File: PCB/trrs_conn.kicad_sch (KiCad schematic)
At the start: 4 parts, among them J501 AudioJack4, J502 AudioJack4, U501 USBLC6-2SC6, U502 USBLC6-2SC6

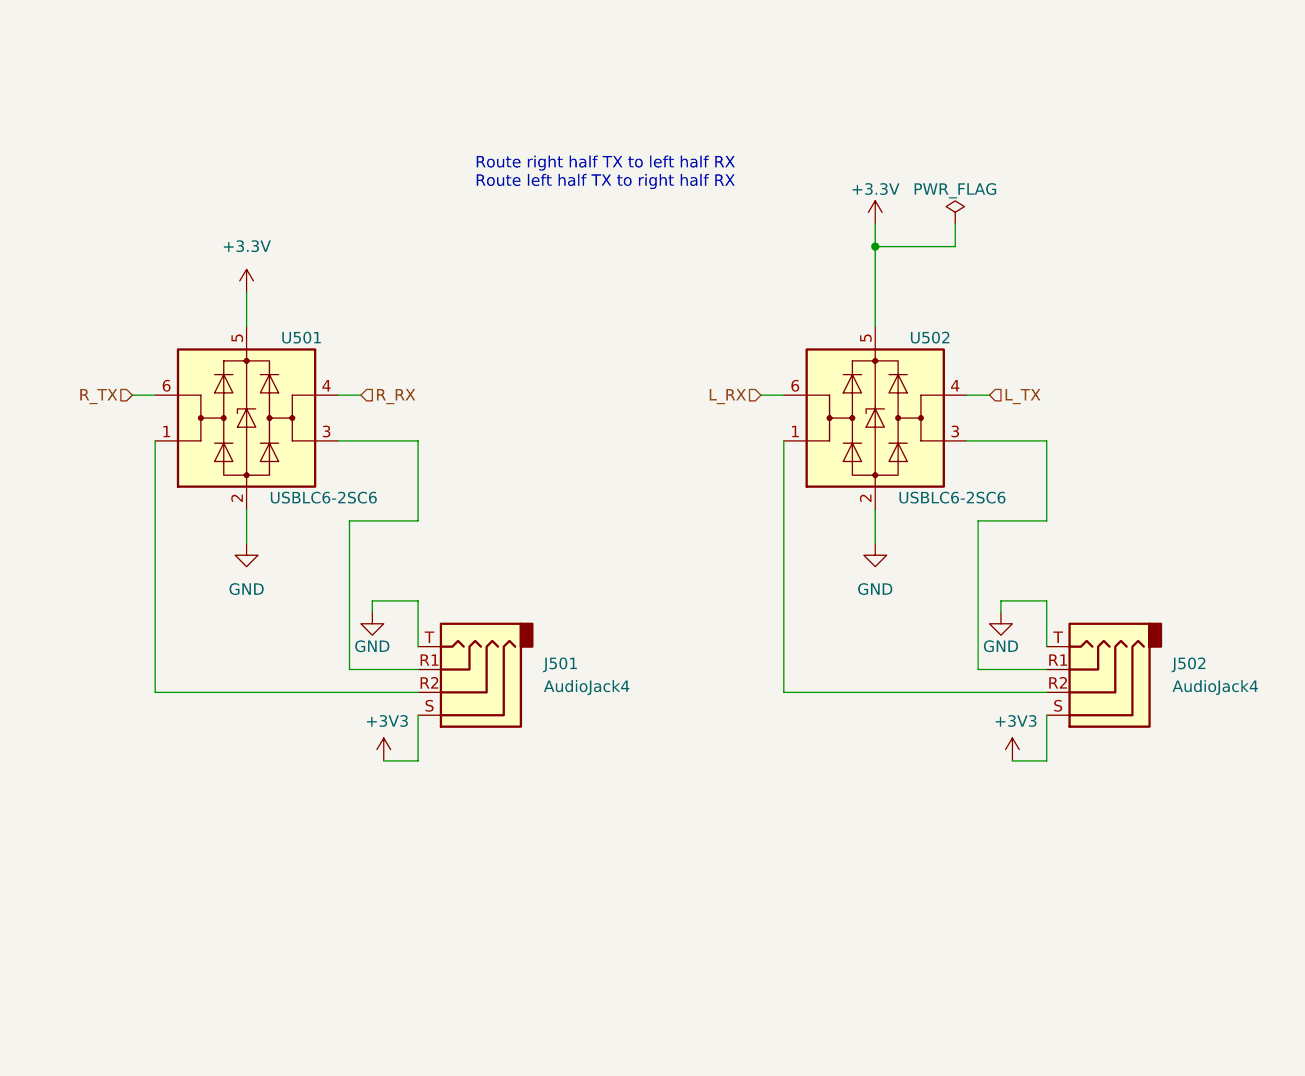
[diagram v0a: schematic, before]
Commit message: Update net labels
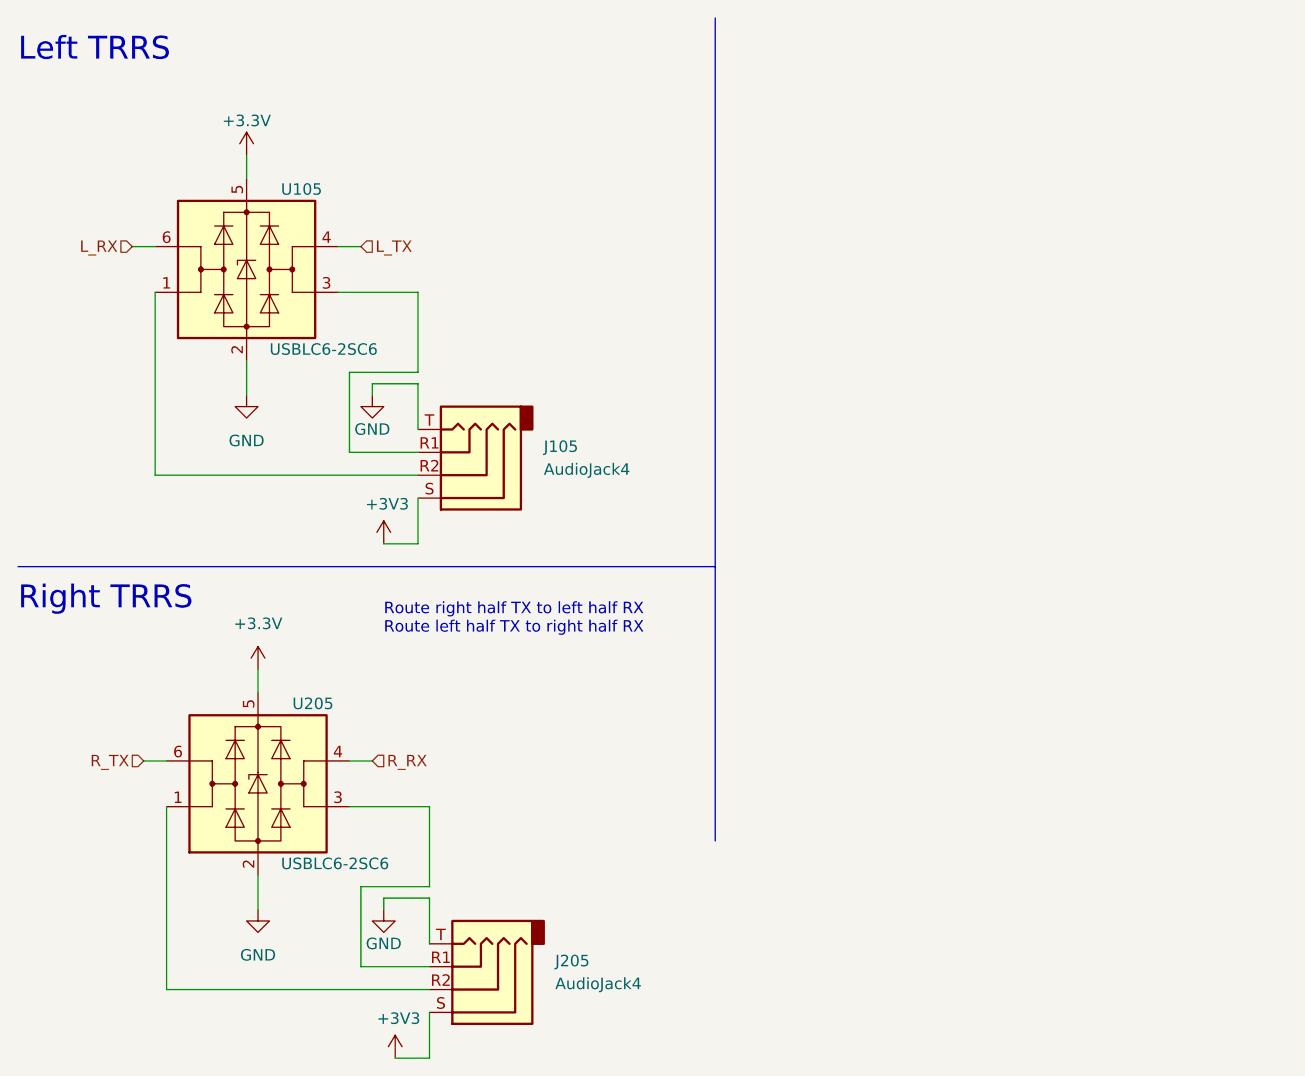
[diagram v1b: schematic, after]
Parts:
- renumbered J502 to J105, J501 to J205, U502 to U105, U501 to U205
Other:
- note added: "Left TRRS"
- note added: "Right TRRS"
- moved on the sheet: J105, J205, U105, U205
